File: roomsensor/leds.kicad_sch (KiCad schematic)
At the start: 25 parts

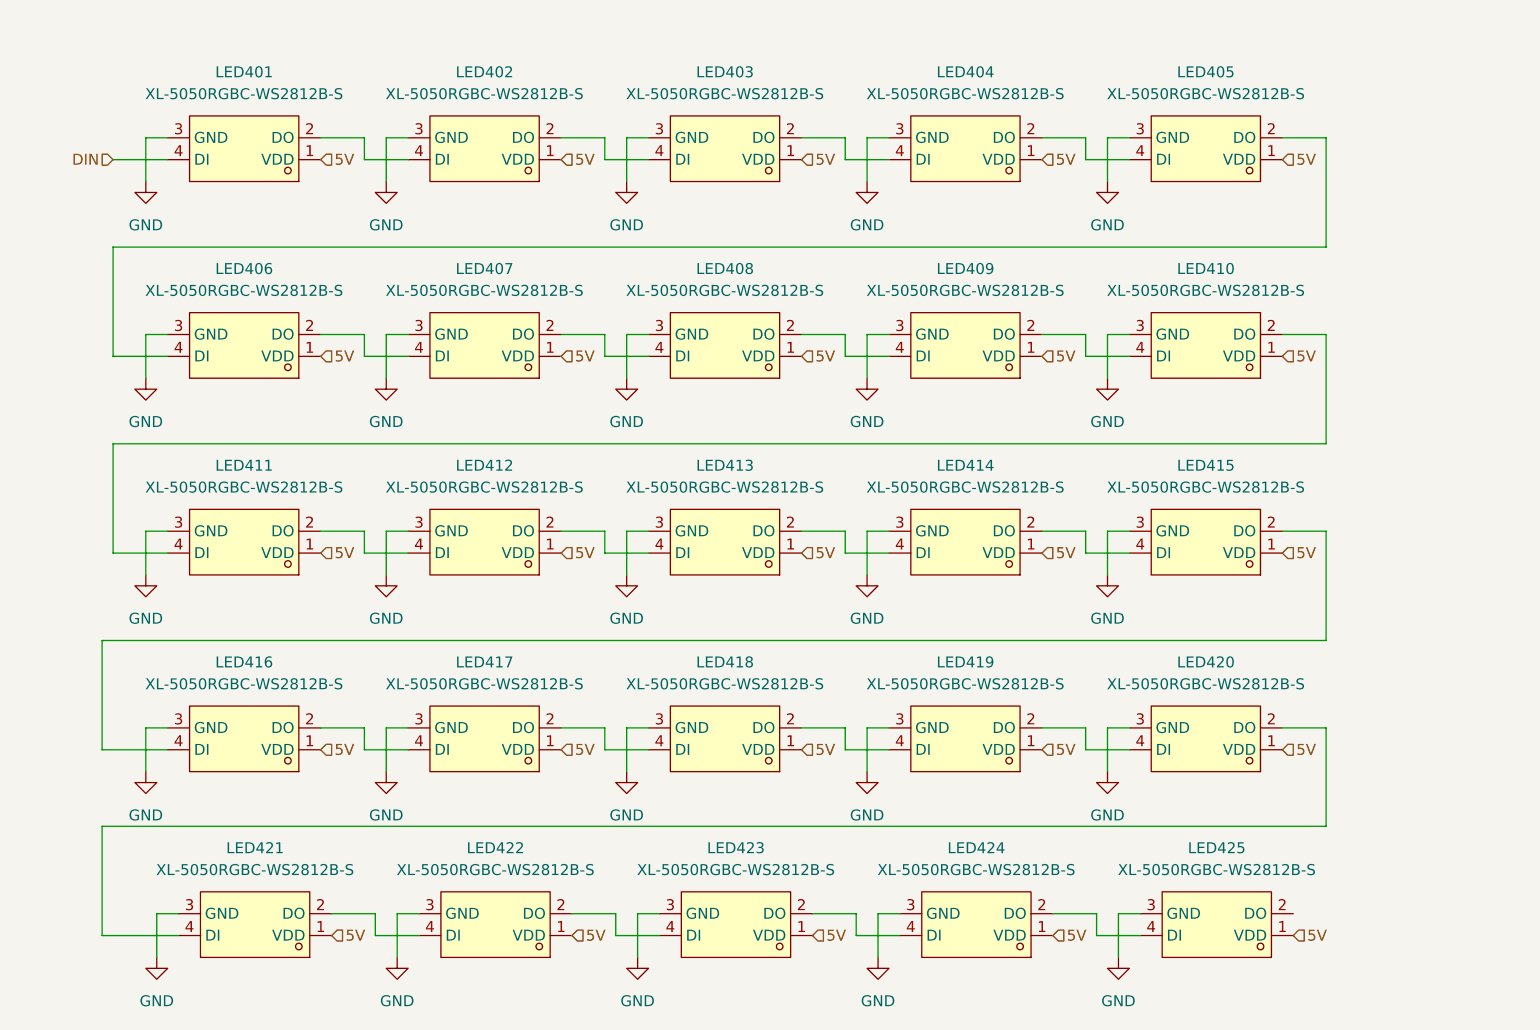
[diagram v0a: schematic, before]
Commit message: sensor v2.1
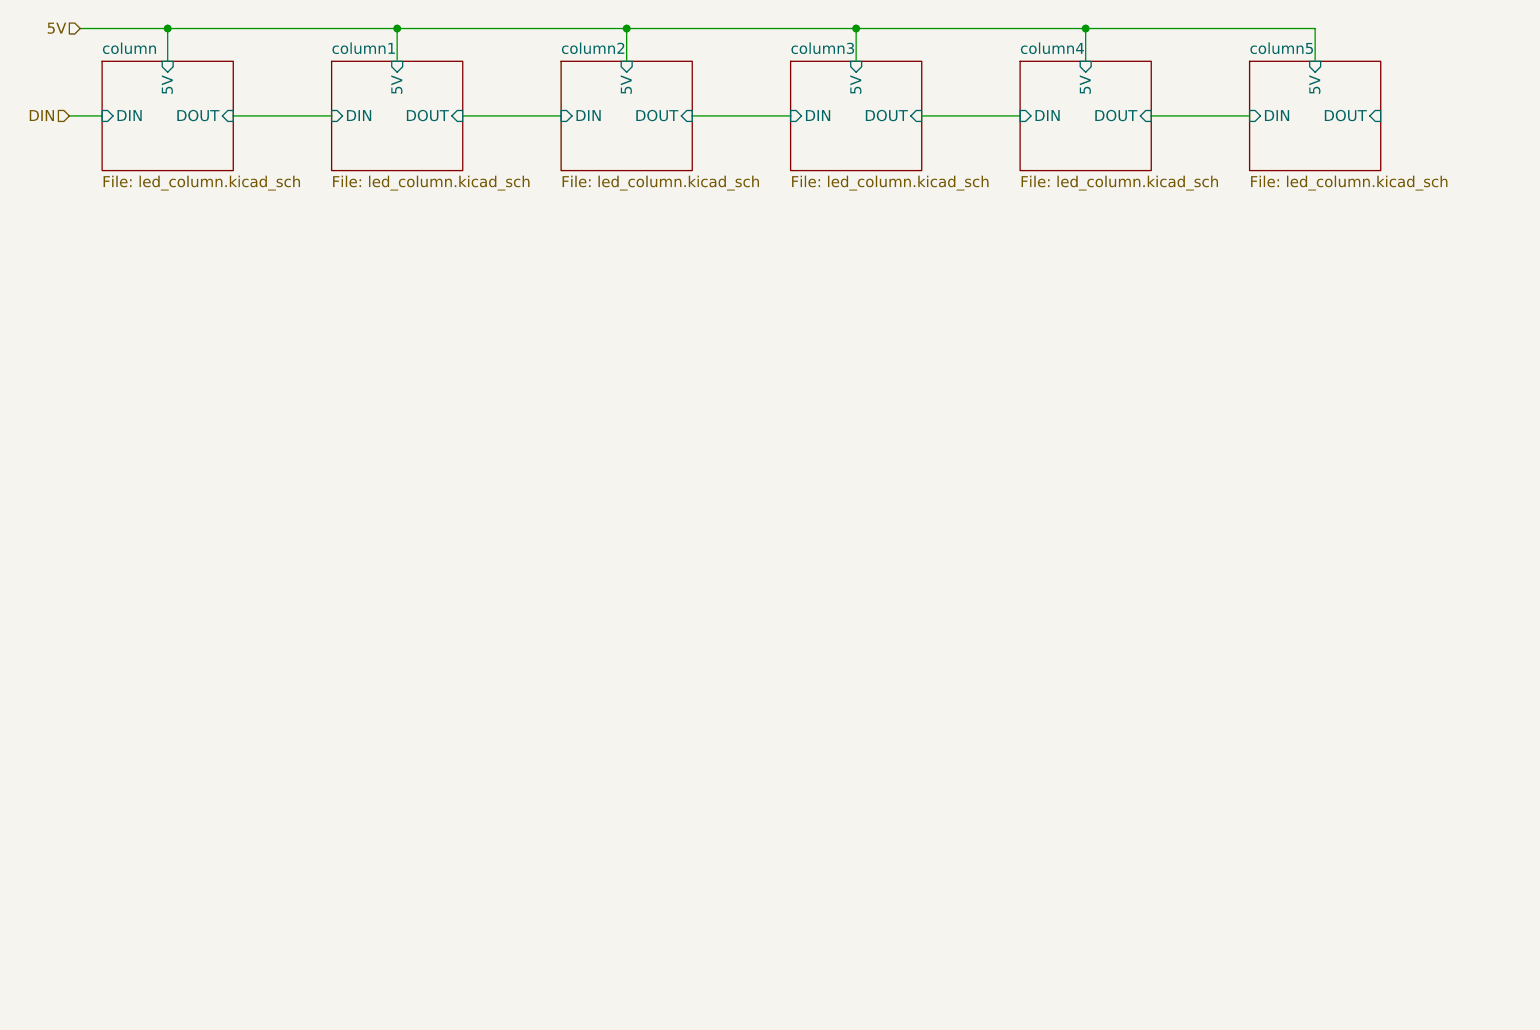
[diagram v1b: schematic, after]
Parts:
- removed LED401, LED402, LED403, LED404, LED405, LED406, LED407, LED408, LED409, LED410, LED411, LED412, LED413, LED414, LED415, LED416, LED417, LED418, LED419, LED420, LED421, LED422, LED423, LED424, LED425: XL-5050RGBC-WS2812B-S, easyeda2kicad:LED-SMD_4P-L5.0-W5.0-TL-1, symbol easyeda2kicad:XL-5050RGBC-WS2812B-S
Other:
- added sheet column (led_column.kicad_sch)
- added sheet column1 (led_column.kicad_sch)
- added sheet column2 (led_column.kicad_sch)
- added sheet column3 (led_column.kicad_sch)
- added sheet column4 (led_column.kicad_sch)
- added sheet column5 (led_column.kicad_sch)
